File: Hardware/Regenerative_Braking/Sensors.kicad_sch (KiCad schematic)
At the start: 46 parts, among them IC4 LM339DT

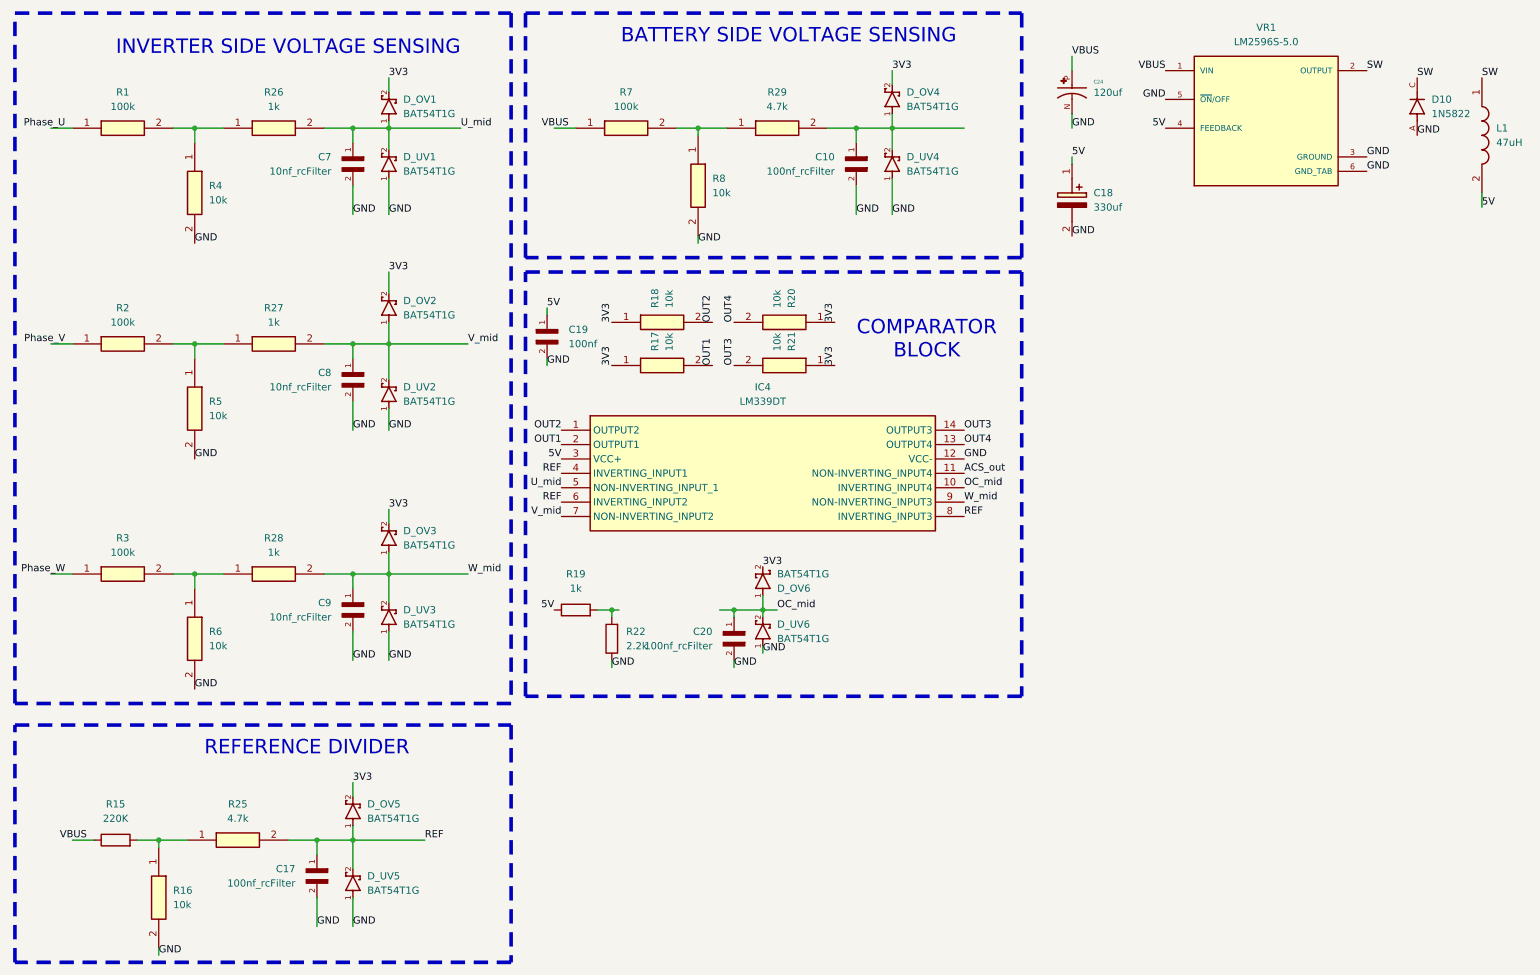
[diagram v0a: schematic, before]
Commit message: finished everything except mcu
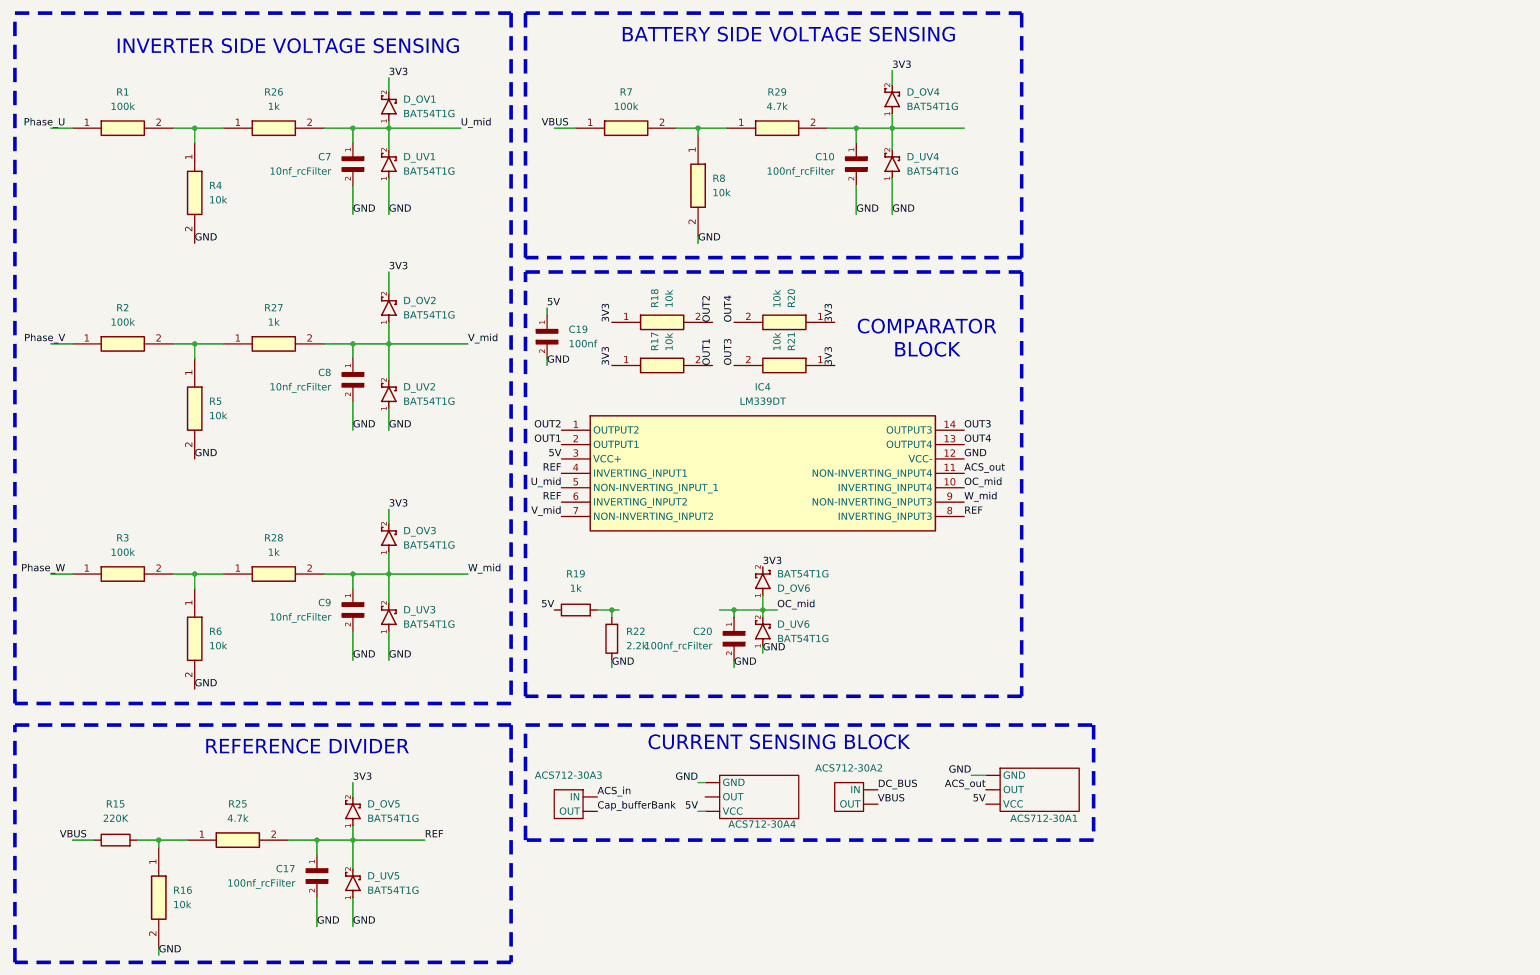
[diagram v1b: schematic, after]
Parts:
- removed C18: 330uf, Regen_braking:330uf_25v_cap_5v_buck, symbol Regen_braking:330uf_25v_cap_5v_buck
- removed C24: 120uf, Regen_braking:120uf_cap_5v_buck, symbol Regen_braking:120uf_cap_5v_buck
- removed D10: 1N5822, Regen_braking:1N5822, symbol Regen_braking:1N5822
- removed L1: 47uH, Regen_braking:47uh_5v_buck, symbol Regen_braking:47uh_5v_buck
- removed VR1: LM2596S-5.0, Regen_braking:5v_buck, symbol Regen_braking:LM2596S-5.0
- added ACS712-30A1, ACS712-30A4: (no value), Regen_braking:ACS712_Module_27x12mm, symbol Regen_braking:ACS712-30A
- added ACS712-30A2, ACS712-30A3: (no value), Regen_braking:Solderpad_acs712_INOUT, symbol Regen_braking:solder_pad_acs712_inout
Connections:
- net 5V: now also ACS712-30A1. (VCC), ACS712-30A4. (VCC)
- net ACS_out: now also ACS712-30A1. (VCC)
- net GND: now also ACS712-30A1. (VCC), ACS712-30A4. (VCC)
- net VBUS: now also ACS712-30A2. (OUT)
- new net ACS_in: ACS712-30A3. (OUT)
- new net Cap_bufferBank: ACS712-30A3. (OUT)
- new net DC_BUS: ACS712-30A2. (OUT)
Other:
- note added: "CURRENT SENSING BLOCK"
